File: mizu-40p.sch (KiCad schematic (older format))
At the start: 14 parts

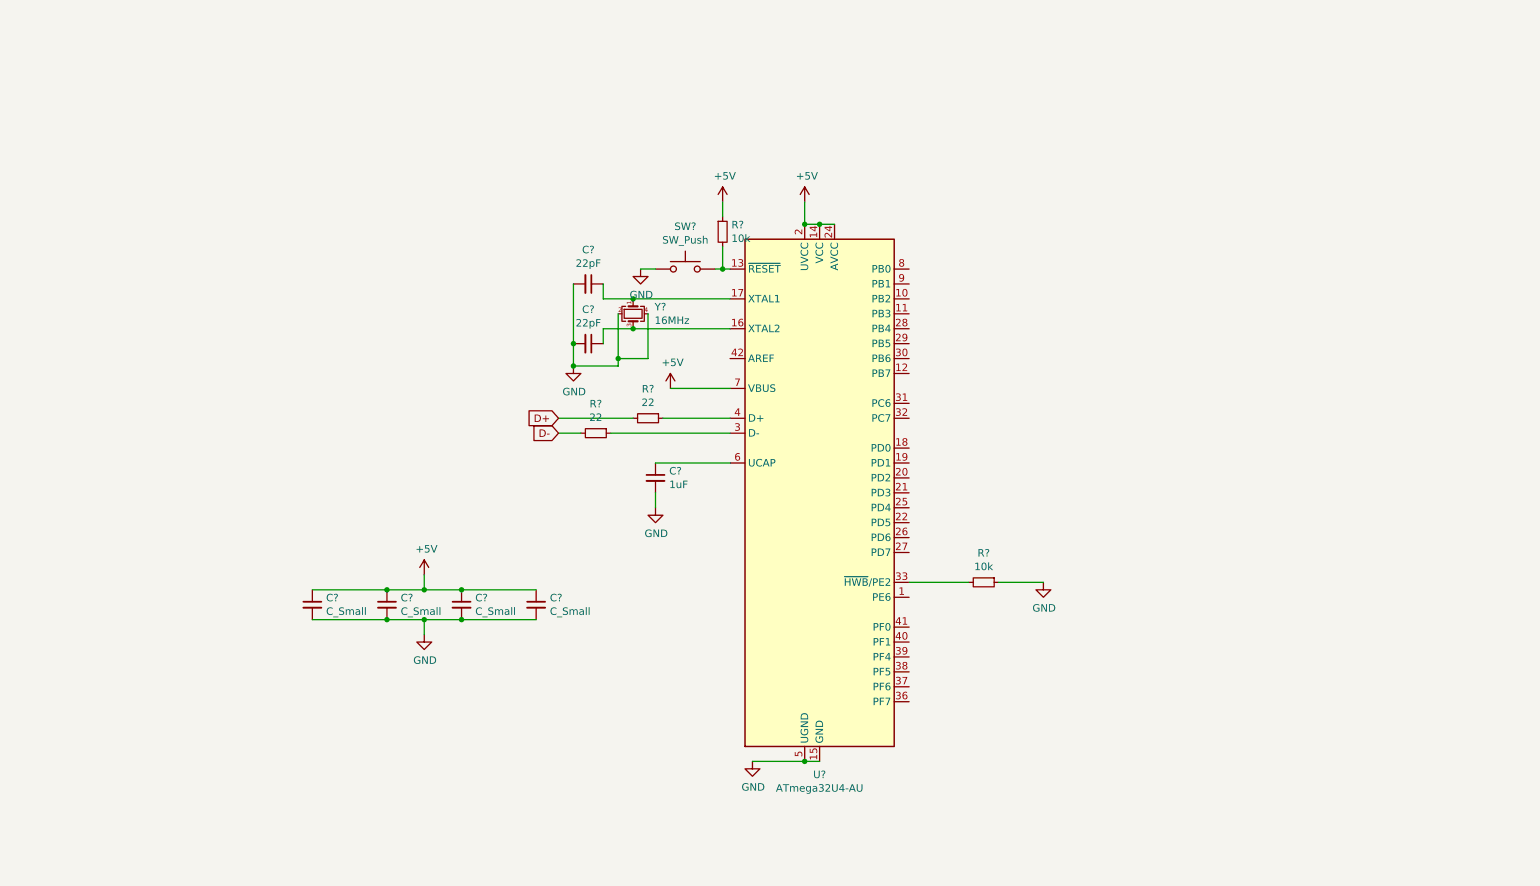
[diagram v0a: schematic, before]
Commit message: Create switch matrix
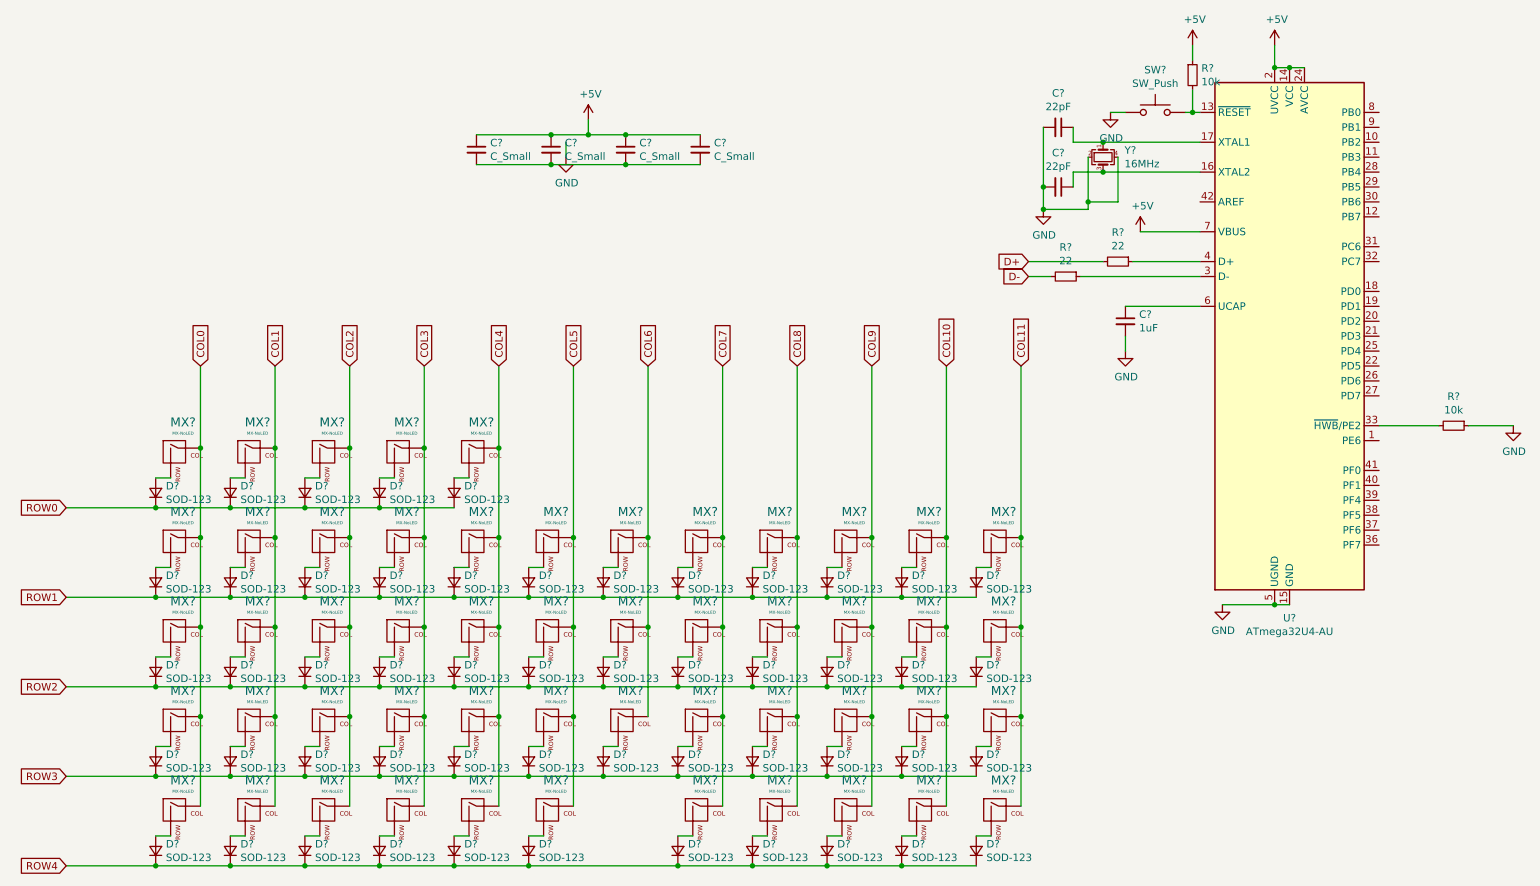
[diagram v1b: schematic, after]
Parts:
- added D? (x52): SOD-123, symbol Device:D_Small
- added MX? (x52): MX-NoLED, symbol MX_Alps_Hybrid:MX-NoLED
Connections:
- net GND: no longer C?.2, C?.2, C?.2, C?.2
- new net: C?.2, C?.2, C?.2, C?.2
- new net: D?.2 (A), MX?.2 (ROW) (x52)
- new net COL0: MX?.1 (COL), MX?.1 (COL), MX?.1 (COL), MX?.1 (COL), MX?.1 (COL)
- new net COL1: MX?.1 (COL), MX?.1 (COL), MX?.1 (COL), MX?.1 (COL), MX?.1 (COL)
- new net COL10: MX?.1 (COL), MX?.1 (COL), MX?.1 (COL), MX?.1 (COL)
- new net COL11: MX?.1 (COL), MX?.1 (COL), MX?.1 (COL), MX?.1 (COL)
- new net COL2: MX?.1 (COL), MX?.1 (COL), MX?.1 (COL), MX?.1 (COL), MX?.1 (COL)
- new net COL3: MX?.1 (COL), MX?.1 (COL), MX?.1 (COL), MX?.1 (COL), MX?.1 (COL)
- new net COL4: MX?.1 (COL), MX?.1 (COL), MX?.1 (COL), MX?.1 (COL), MX?.1 (COL)
- new net COL5: MX?.1 (COL), MX?.1 (COL), MX?.1 (COL), MX?.1 (COL)
- new net COL6: MX?.1 (COL), MX?.1 (COL), MX?.1 (COL)
- new net COL7: MX?.1 (COL), MX?.1 (COL), MX?.1 (COL), MX?.1 (COL)
- new net COL8: MX?.1 (COL), MX?.1 (COL), MX?.1 (COL), MX?.1 (COL)
- new net COL9: MX?.1 (COL), MX?.1 (COL), MX?.1 (COL), MX?.1 (COL)
- new net ROW0: D?.1 (K), D?.1 (K), D?.1 (K), D?.1 (K), D?.1 (K)
- new net ROW1: D?.1 (K), D?.1 (K), D?.1 (K), D?.1 (K), D?.1 (K), D?.1 (K), D?.1 (K), D?.1 (K), D?.1 (K), D?.1 (K), D?.1 (K), D?.1 (K)
- new net ROW2: D?.1 (K), D?.1 (K), D?.1 (K), D?.1 (K), D?.1 (K), D?.1 (K), D?.1 (K), D?.1 (K), D?.1 (K), D?.1 (K), D?.1 (K), D?.1 (K)
- new net ROW3: D?.1 (K), D?.1 (K), D?.1 (K), D?.1 (K), D?.1 (K), D?.1 (K), D?.1 (K), D?.1 (K), D?.1 (K), D?.1 (K), D?.1 (K), D?.1 (K)
- new net ROW4: D?.1 (K), D?.1 (K), D?.1 (K), D?.1 (K), D?.1 (K), D?.1 (K), D?.1 (K), D?.1 (K), D?.1 (K), D?.1 (K), D?.1 (K)
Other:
- moved on the sheet: C?, R?, SW?, U?, Y?
